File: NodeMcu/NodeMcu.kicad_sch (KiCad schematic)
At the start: 38 parts, among them J1 Conn_01x15_Male, J2 Conn_01x15_Male, P1 USB_C_Plug_USB2.0, Q1 Q_Dual_NPN_NPN_E1B1C2E2B2C1, SW1 SW_Push, SW2 SW_Push, U1 ESP-12E, U2 SPX3819M5-L-3-3, U3 CH340C

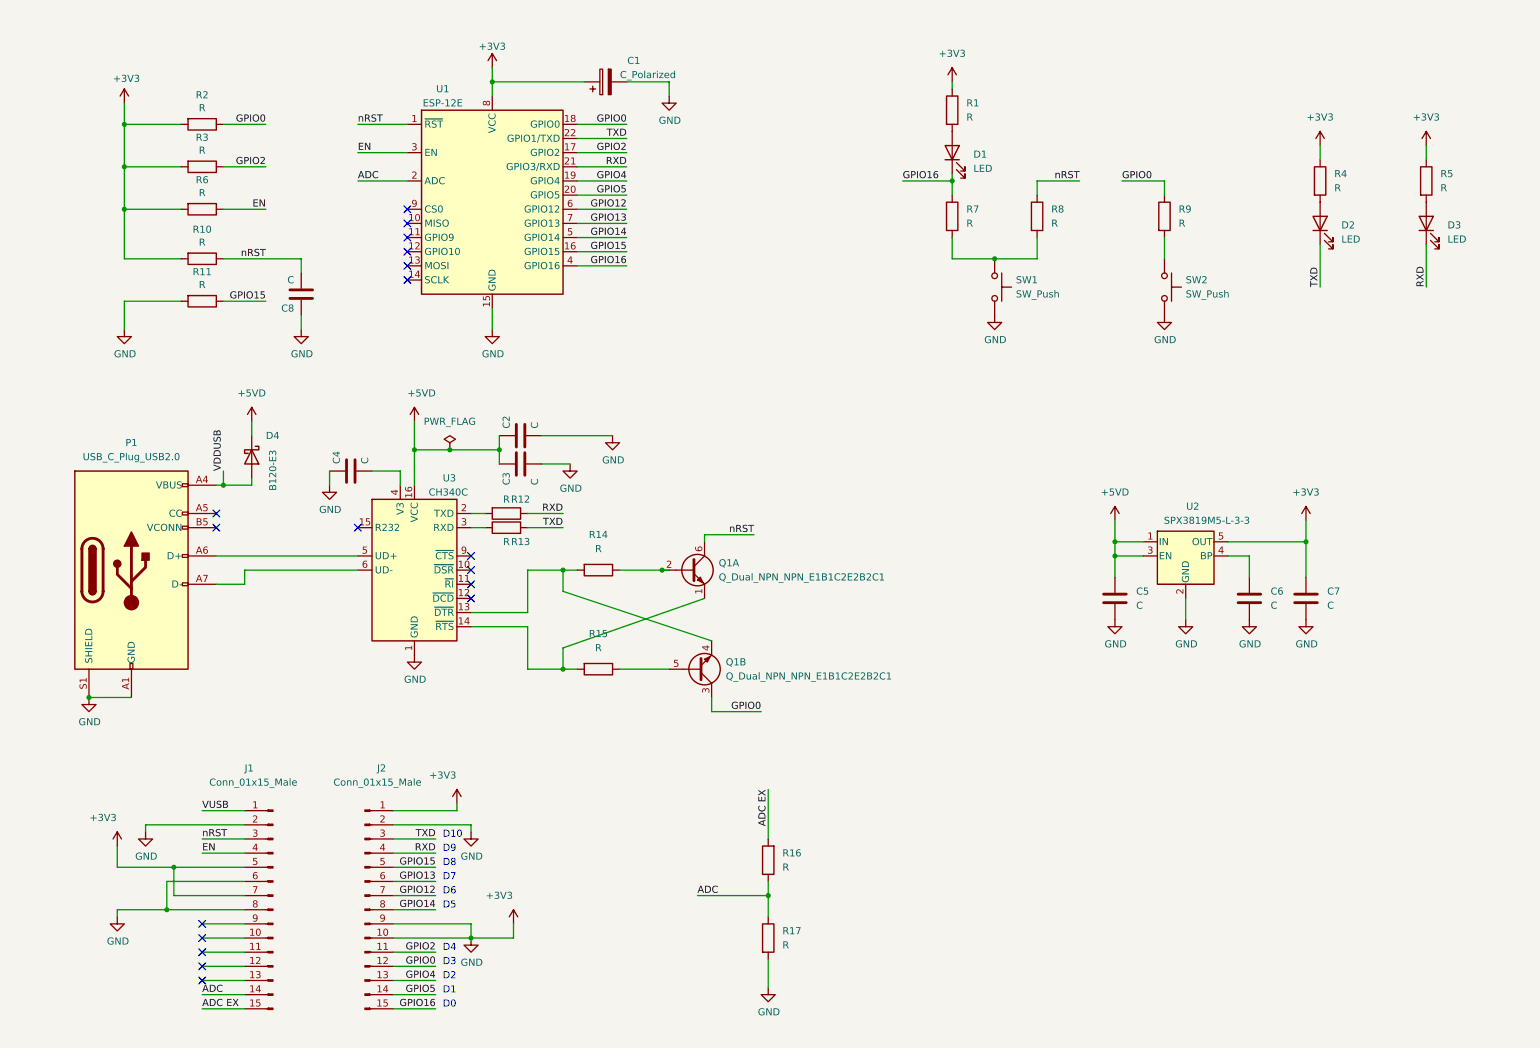
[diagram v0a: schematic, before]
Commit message: nodemcu
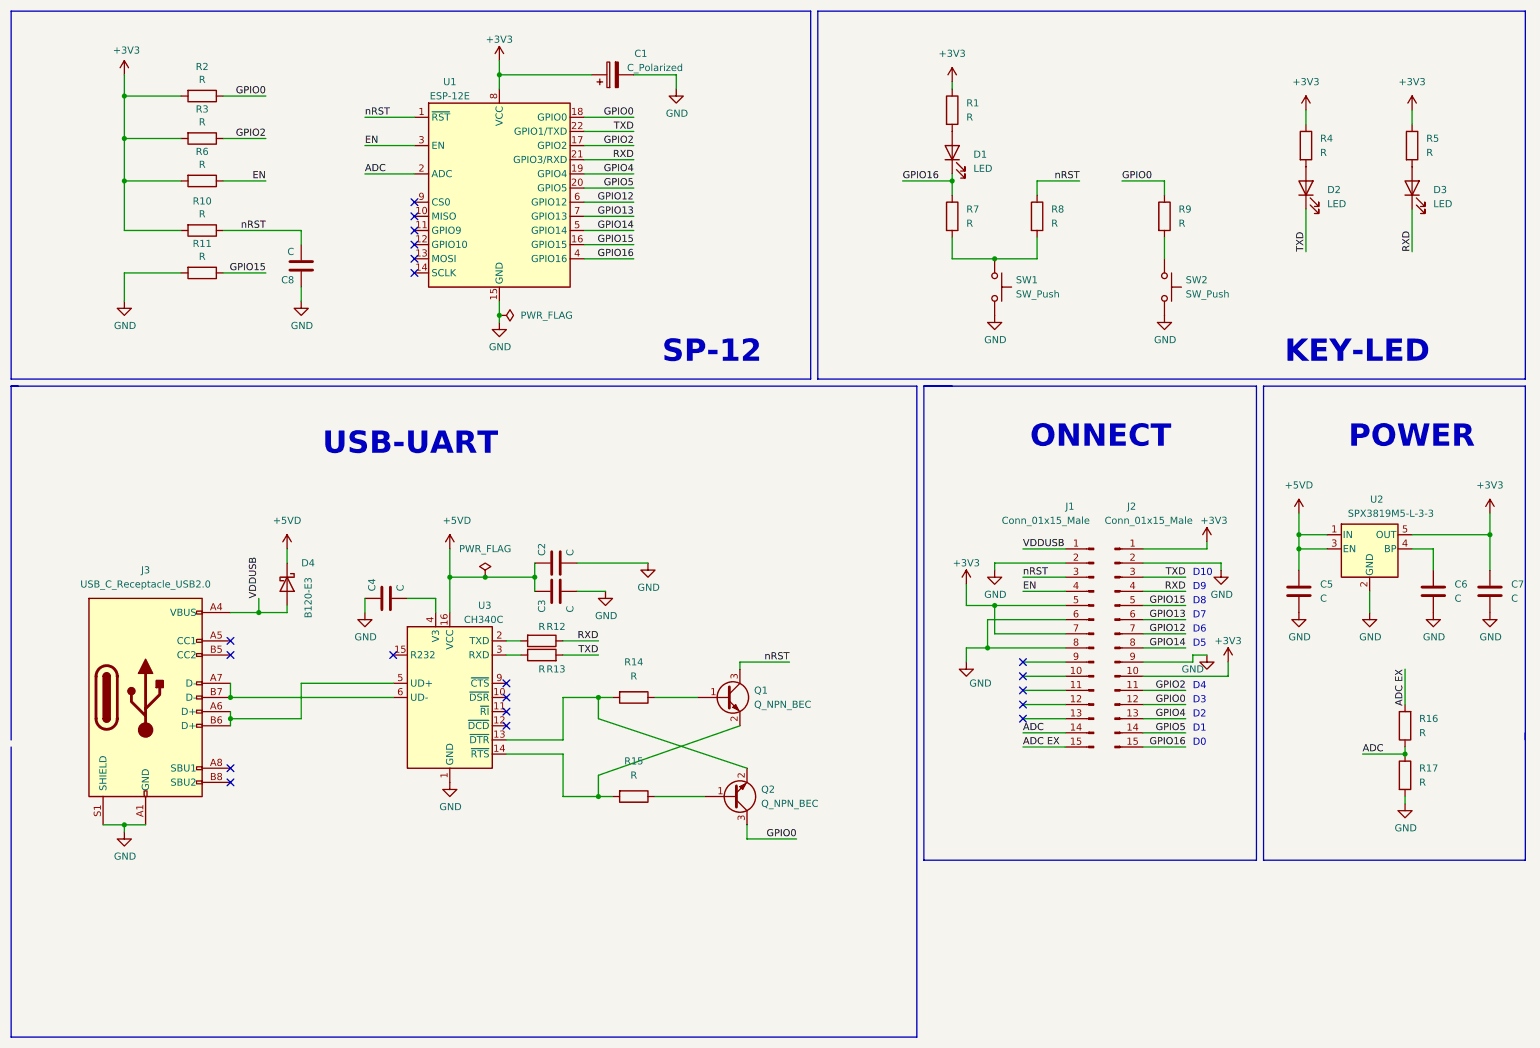
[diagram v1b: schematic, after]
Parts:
- removed P1: USB_C_Plug_USB2.0, Connector_USB:USB_C_Plug_JAE_DX07P024AJ1, symbol Connector:USB_C_Plug_USB2.0
- removed Q1: Q_Dual_NPN_NPN_E1B1C2E2B2C1, Package_TO_SOT_SMD:SOT-23, symbol Device:Q_Dual_NPN_NPN_E1B1C2E2B2C1
- added J3: USB_C_Receptacle_USB2.0, Connector_USB:USB_C_Receptacle_HRO_TYPE-C-31-M-12, symbol Connector:USB_C_Receptacle_USB2.0
- added Q1, Q2: Q_NPN_BEC, Package_TO_SOT_SMD:SOT-23, symbol Device:Q_NPN_BEC
- J1, J2: footprint Connector_DIN:DIN41612_B_1x32_Male_Horizontal_THT -> Connector_PinHeader_2.54mm:PinHeader_1x15_P2.54mm_Vertical
- SW1, SW2: footprint Button_Switch_THT:SW_PUSH_6mm -> Button_Switch_SMD:SW_SPST_FSMSM
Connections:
- net VUSB is gone; now on net VDDUSB: J1.1 (Pin_1)
- net +3V3: no longer C1.2, C2.2, C3.2, C4.1, C5.2, C6.2, C7.2, C8.1, J1.2 (Pin_2), J1.6 (Pin_6), J1.8 (Pin_8), J2.2 (Pin_2), J2.9 (Pin_9), R11.2, R17.2, SW1.2, SW2.2, U1.15 (GND), U2.2 (GND), U3.1 (GND)
- net GPIO0: now also Q2.3 (C)
- net VDDUSB: now also J3.A4 (VBUS), J3.A9 (VBUS), J3.B4 (VBUS), J3.B9 (VBUS)
- net nRST: now also Q1.3 (C)
- net at R14.2, U3.13 (~{DTR}): now also Q2.2 (E)
- net at R15.2, U3.14 (~{RTS}): now also Q1.2 (E)
- net at U3.5 (UD+): now also J3.A6 (D+), J3.B6 (D+)
- net at U3.6 (UD-): now also J3.A7 (D-), J3.B7 (D-)
- net at R15.1: now also Q2.1 (B)
- net at R14.1: now also Q1.1 (B)
- new net GND: C1.2, C2.2, C3.2, C4.1, C5.2, C6.2, C7.2, C8.1, J1.2 (Pin_2), J1.6 (Pin_6), J1.8 (Pin_8), J2.2 (Pin_2), J2.9 (Pin_9), J3.A1 (GND), J3.A12 (GND), J3.B1 (GND), J3.B12 (GND), J3.S1 (SHIELD), R11.2, R17.2, SW1.2, SW2.2, U1.15 (GND), U2.2 (GND), U3.1 (GND)
- no-connect marks 18 -> 20
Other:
- note added: "KEY-LED"
- note added: "ONNECT"
- note added: "POWER"
- note added: "SP-12"
- note added: "USB-UART"
- moved on the sheet: C1, C2, C3, C4, C5, C6, C7, C8, D2, D3, D4, J1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
